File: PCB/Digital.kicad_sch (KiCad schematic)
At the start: 16 parts, among them IC1 MAX3051ESA+, J2 ICSP, J3 DE9_Plug_MountingHoles, J4 Conn_Coaxial, J5 DE9_Plug_MountingHoles, U1 PIC18F2580T-I/SO, Y2 ABLS-8.000MHZ-B2-T

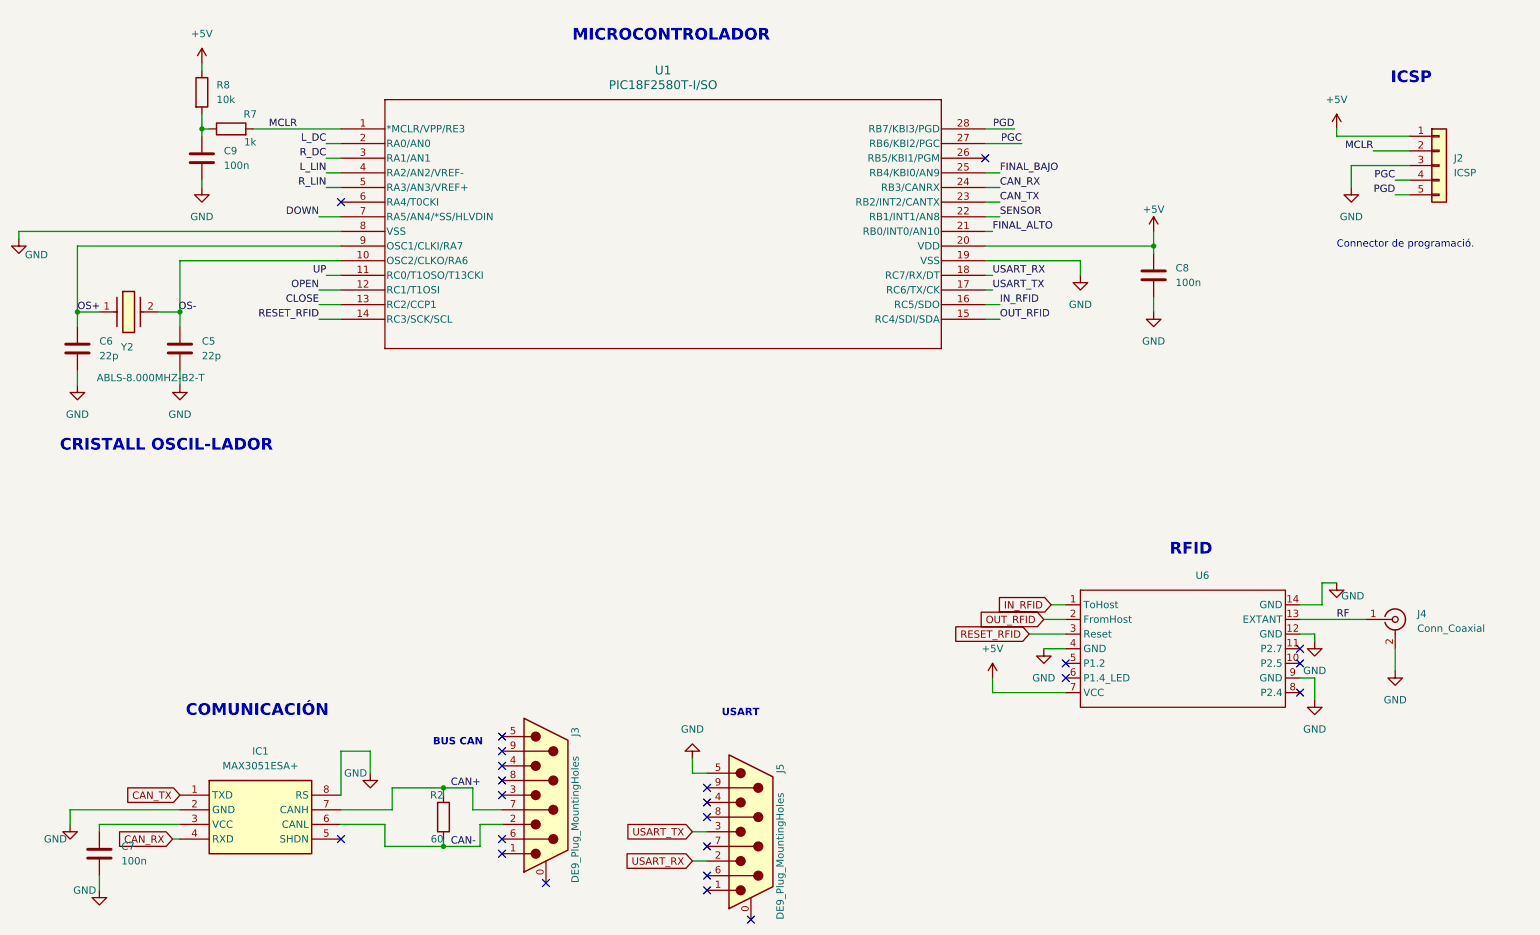
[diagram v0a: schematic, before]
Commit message: Update Digital.kicad_sch
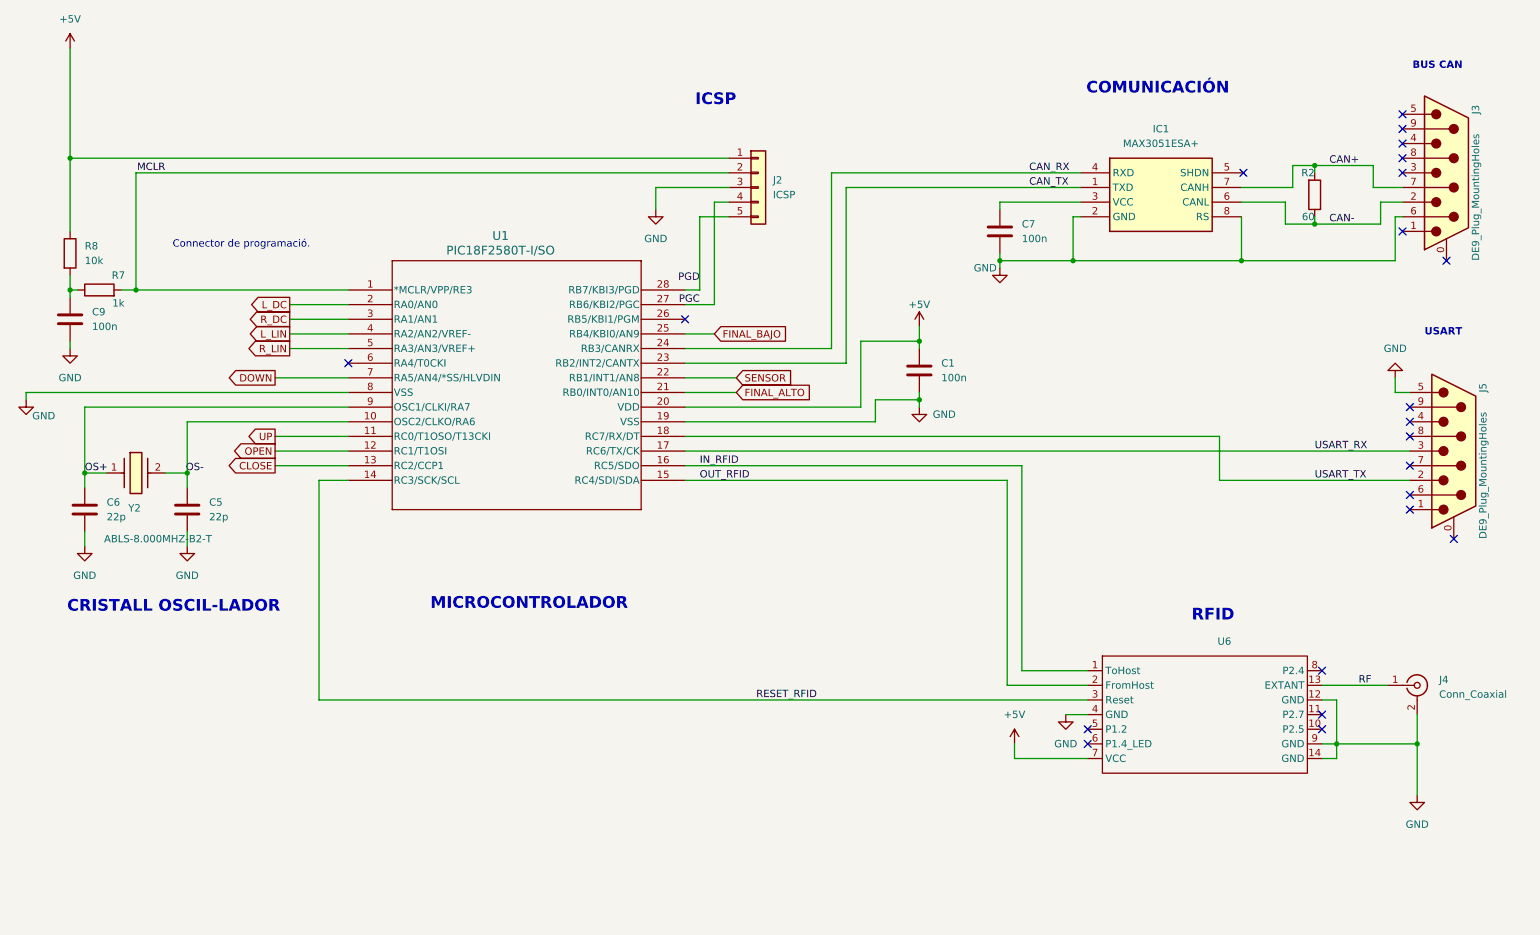
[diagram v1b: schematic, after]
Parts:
- removed C8: 100n, symbol Device:C
- added C1: 100n, symbol Device:C
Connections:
- net +5V: now also C1.1
- net GND: now also J3.6, C1.2
- net USART_RX: now also J5.3, U1.17 (RC6/TX/CK); no longer J5.2, U1.18 (RC7/RX/DT)
- net USART_TX: now also J5.2, U1.18 (RC7/RX/DT); no longer J5.3, U1.17 (RC6/TX/CK)
- no-connect marks 23 -> 22
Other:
- moved on the sheet: C5, C6, C7, C9, IC1, J2, J3, J4, J5, R2, R7, R8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
